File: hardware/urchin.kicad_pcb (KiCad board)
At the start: 2 copper layers, 19 parts, among them IC1 ATMEGA328PB-A, IC2 ATTINY85-S, P1 CONN_02X03, P2 USB_OTG, U1 CH340G, Y1 12M

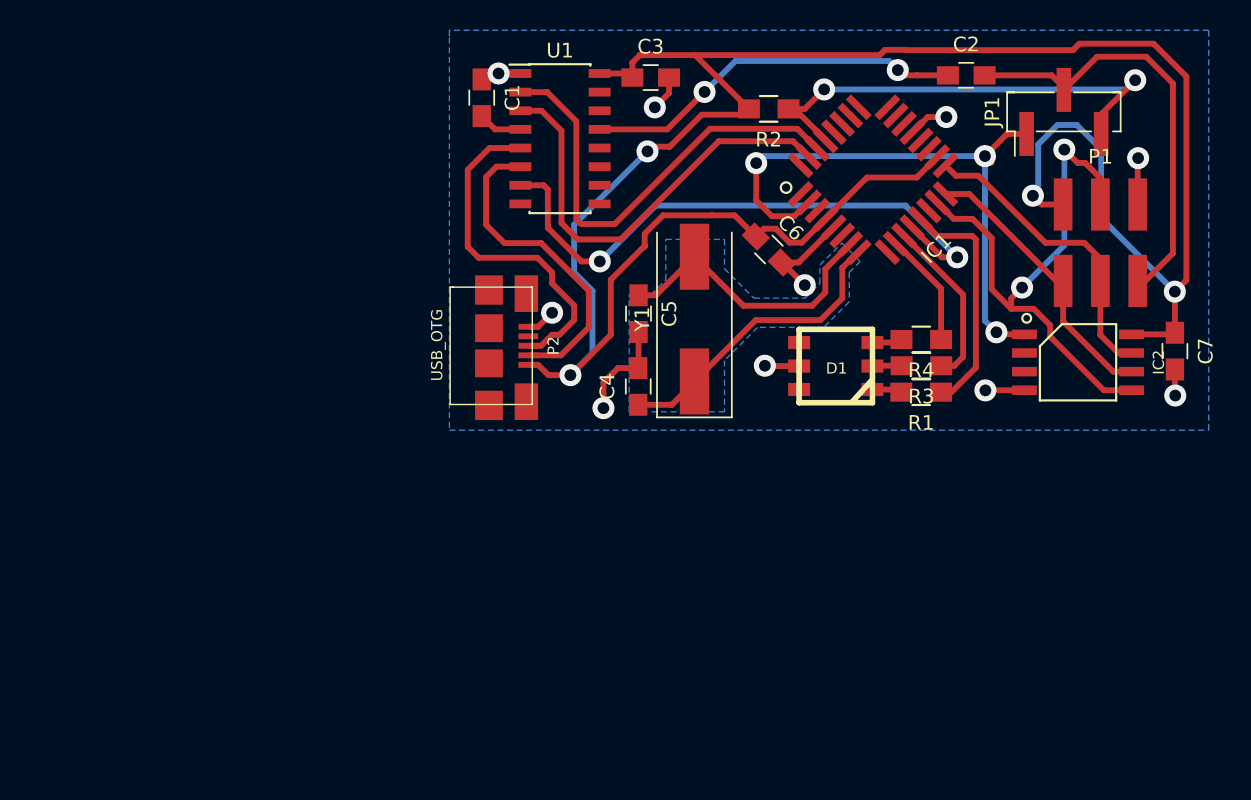
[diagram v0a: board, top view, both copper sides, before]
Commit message: Centering
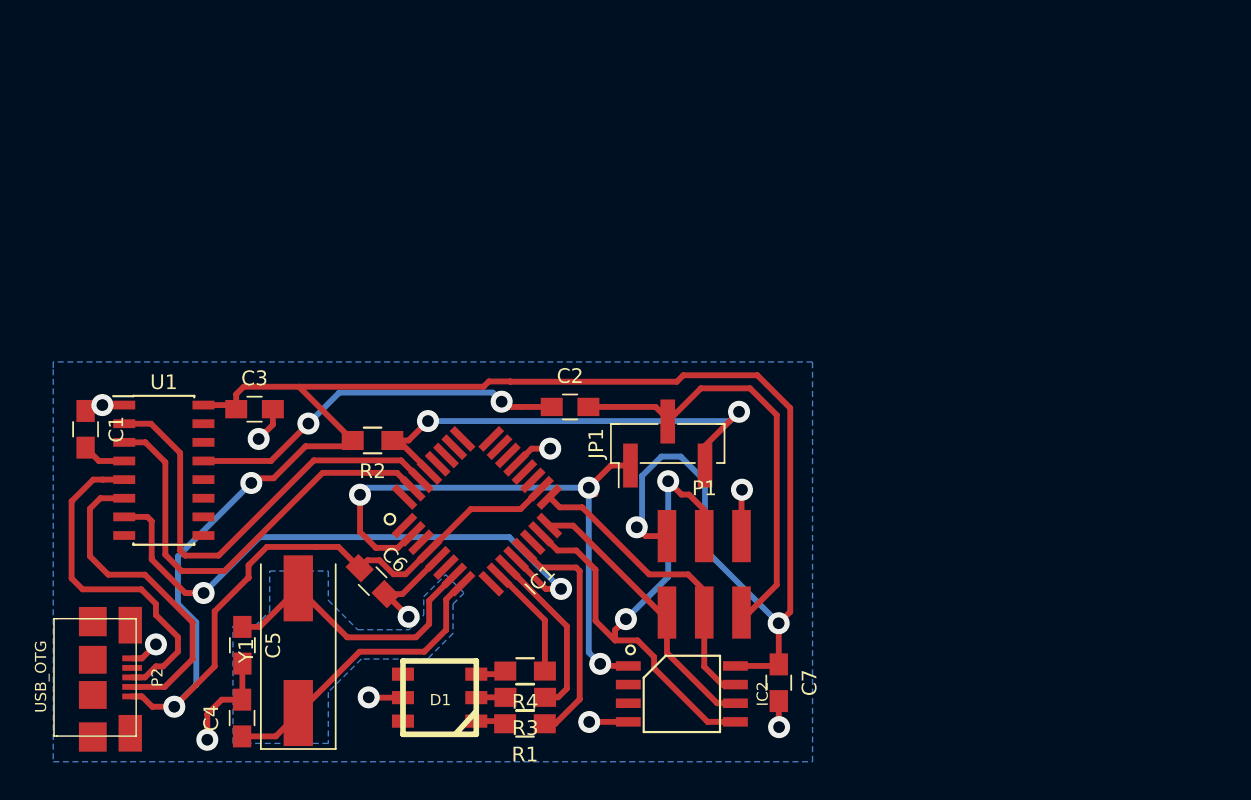
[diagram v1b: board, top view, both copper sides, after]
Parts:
- moved U1 35.2 mm to (118.3, 94.7)
- moved C1 35.2 mm to (113.0, 91.9)
- moved C2 35.2 mm to (146.0, 90.4)
- moved C4 35.2 mm to (123.6, 111.6)
- moved C6 35.2 mm to (132.5, 102.3)
- moved D1 35.2 mm to (137.1, 110.2)
- moved R1 35.2 mm to (142.9, 112.0)
- moved R4 35.2 mm to (142.9, 108.4)
- moved C3 35.2 mm to (124.5, 90.6)
- moved C7 35.2 mm to (160.2, 109.2)
- moved IC1 35.2 mm to (139.6, 97.5)
- moved IC2 35.2 mm to (153.6, 110.0)
- moved JP1 35.2 mm to (152.6, 92.9)
- moved P1 35.2 mm to (155.1, 102.6)
- moved P2 35.2 mm to (112.0, 108.8)
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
